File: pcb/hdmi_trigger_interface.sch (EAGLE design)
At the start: 58 parts, among them U1 TPD12S016PWR, U2 TPD12S016PWR, Y1 SI514

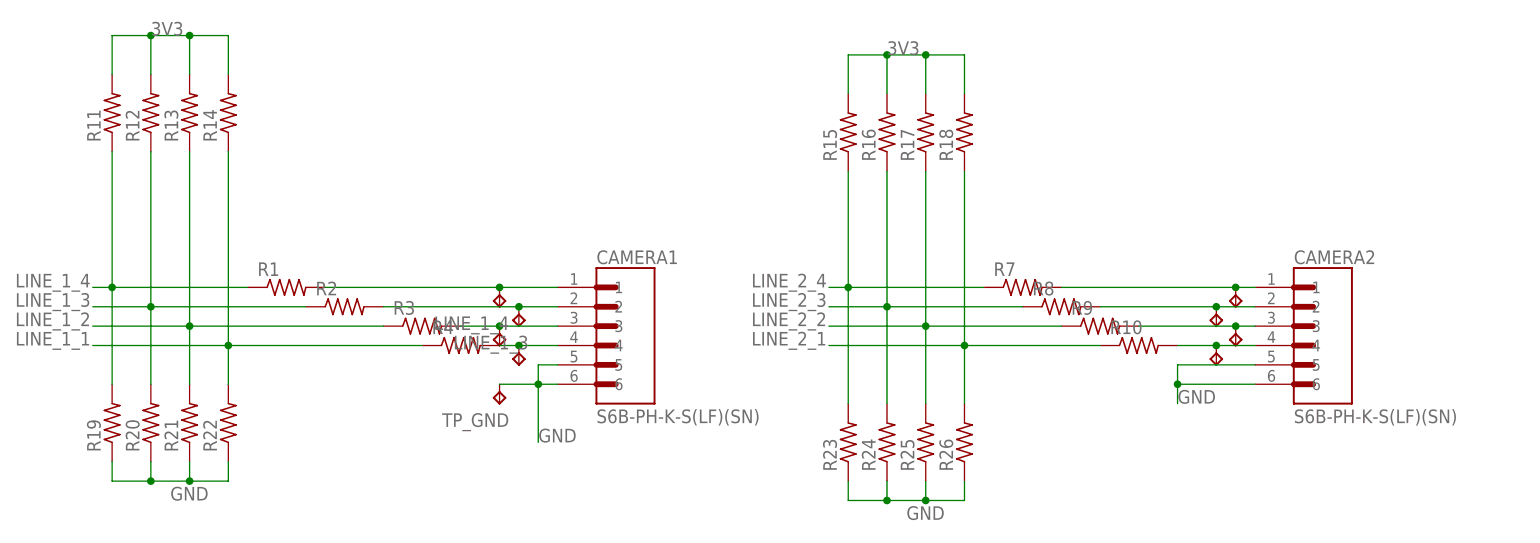
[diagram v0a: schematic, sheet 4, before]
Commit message: more routing
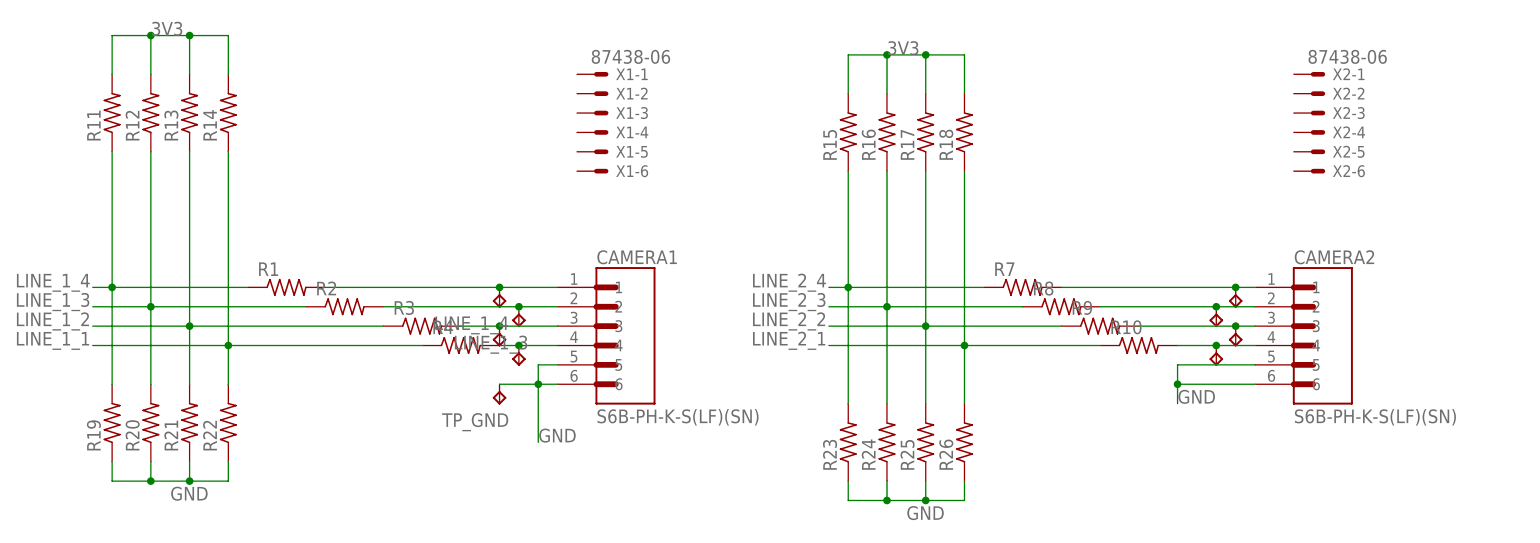
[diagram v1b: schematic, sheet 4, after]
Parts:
- added X1, X2: 87438-06, con-molex:87438-06
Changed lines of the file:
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@@
 <part name="CAMERA1" library="S6B-PH-K-S_LF__SN_" deviceset="S6B-PH-K-S(LF)(SN)" device=""/>
 <part name="CAMERA2" library="S6B-PH-K-S_LF__SN_" deviceset="S6B-PH-K-S(LF)(SN)" device=""/>
+<part name="X1" library="con-molex" library_urn="urn:adsk.eagle:library:165" deviceset="87438-06" device="" package3d_urn="urn:adsk.eagle:package:8078913/1"/>
+<part name="X2" library="con-molex" library_urn="urn:adsk.eagle:library:165" deviceset="87438-06" device="" package3d_urn="urn:adsk.eagle:package:8078913/1"/>
 </parts>
 <sheets>
@@
 <attribute name="VALUE" x="177.8" y="22.8446" size="1.780159375" layer="96"/>
 </instance>
+<instance part="X1" gate="-1" x="86.36" y="68.58" smashed="yes">
+<attribute name="NAME" x="88.9" y="67.818" size="1.524" layer="95"/>
+<attribute name="VALUE" x="85.598" y="69.977" size="1.778" layer="96"/>
+</instance>
+<instance part="X1" gate="-2" x="86.36" y="66.04" smashed="yes">
+<attribute name="NAME" x="88.9" y="65.278" size="1.524" layer="95"/>
+</instance>
+<instance part="X1" gate="-3" x="86.36" y="63.5" smashed="yes">
+<attribute name="NAME" x="88.9" y="62.738" size="1.524" layer="95"/>
+</instance>
+<instance part="X1" gate="-4" x="86.36" y="60.96" smashed="yes">
+<attribute name="NAME" x="88.9" y="60.198" size="1.524" layer="95"/>
+</instance>
+<instance part="X1" gate="-5" x="86.36" y="58.42" smashed="yes">
+<attribute name="NAME" x="88.9" y="57.658" size="1.524" layer="95"/>
+</instance>
+<instance part="X1" gate="-6" x="86.36" y="55.88" smashed="yes">
+<attribute name="NAME" x="88.9" y="55.118" size="1.524" layer="95"/>
+</instance>
+<instance part="X2" gate="-1" x="180.34" y="68.58" smashed="yes">
+<attribute name="NAME" x="182.88" y="67.818" size="1.524" layer="95"/>
+<attribute name="VALUE" x="179.578" y="69.977" size="1.778" layer="96"/>
+</instance>
+<instance part="X2" gate="-2" x="180.34" y="66.04" smashed="yes">
+<attribute name="NAME" x="182.88" y="65.278" size="1.524" layer="95"/>
+</instance>
+<instance part="X2" gate="-3" x="180.34" y="63.5" smashed="yes">
+<attribute name="NAME" x="182.88" y="62.738" size="1.524" layer="95"/>
+</instance>
+<instance part="X2" gate="-4" x="180.34" y="60.96" smashed="yes">
+<attribute name="NAME" x="182.88" y="60.198" size="1.524" layer="95"/>
+</instance>
+<instance part="X2" gate="-5" x="180.34" y="58.42" smashed="yes">
+<attribute name="NAME" x="182.88" y="57.658" size="1.524" layer="95"/>
+</instance>
+<instance part="X2" gate="-6" x="180.34" y="55.88" smashed="yes">
+<attribute name="NAME" x="182.88" y="55.118" size="1.524" layer="95"/>
+</instance>
 </instances>
